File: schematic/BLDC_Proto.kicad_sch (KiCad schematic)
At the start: 50 parts, among them J1 Motor Encoder In, M1 Hobbywing QuicRun 3650, Q1 GSFN0390, Q2 GSFN0390, Q3 GSFN0390, Q4 GSFN0390, Q5 GSFN0390, Q6 GSFN0390, SW1 SW_Push, SW2 Keypad, U1 ESP32-S3-DevKitC, U2 AP62200TWU, U3 DRV8300D, U4 74HC595, U5 74HC595, U6 BA56-12SURKWA, U7 BA56-12SURKWA

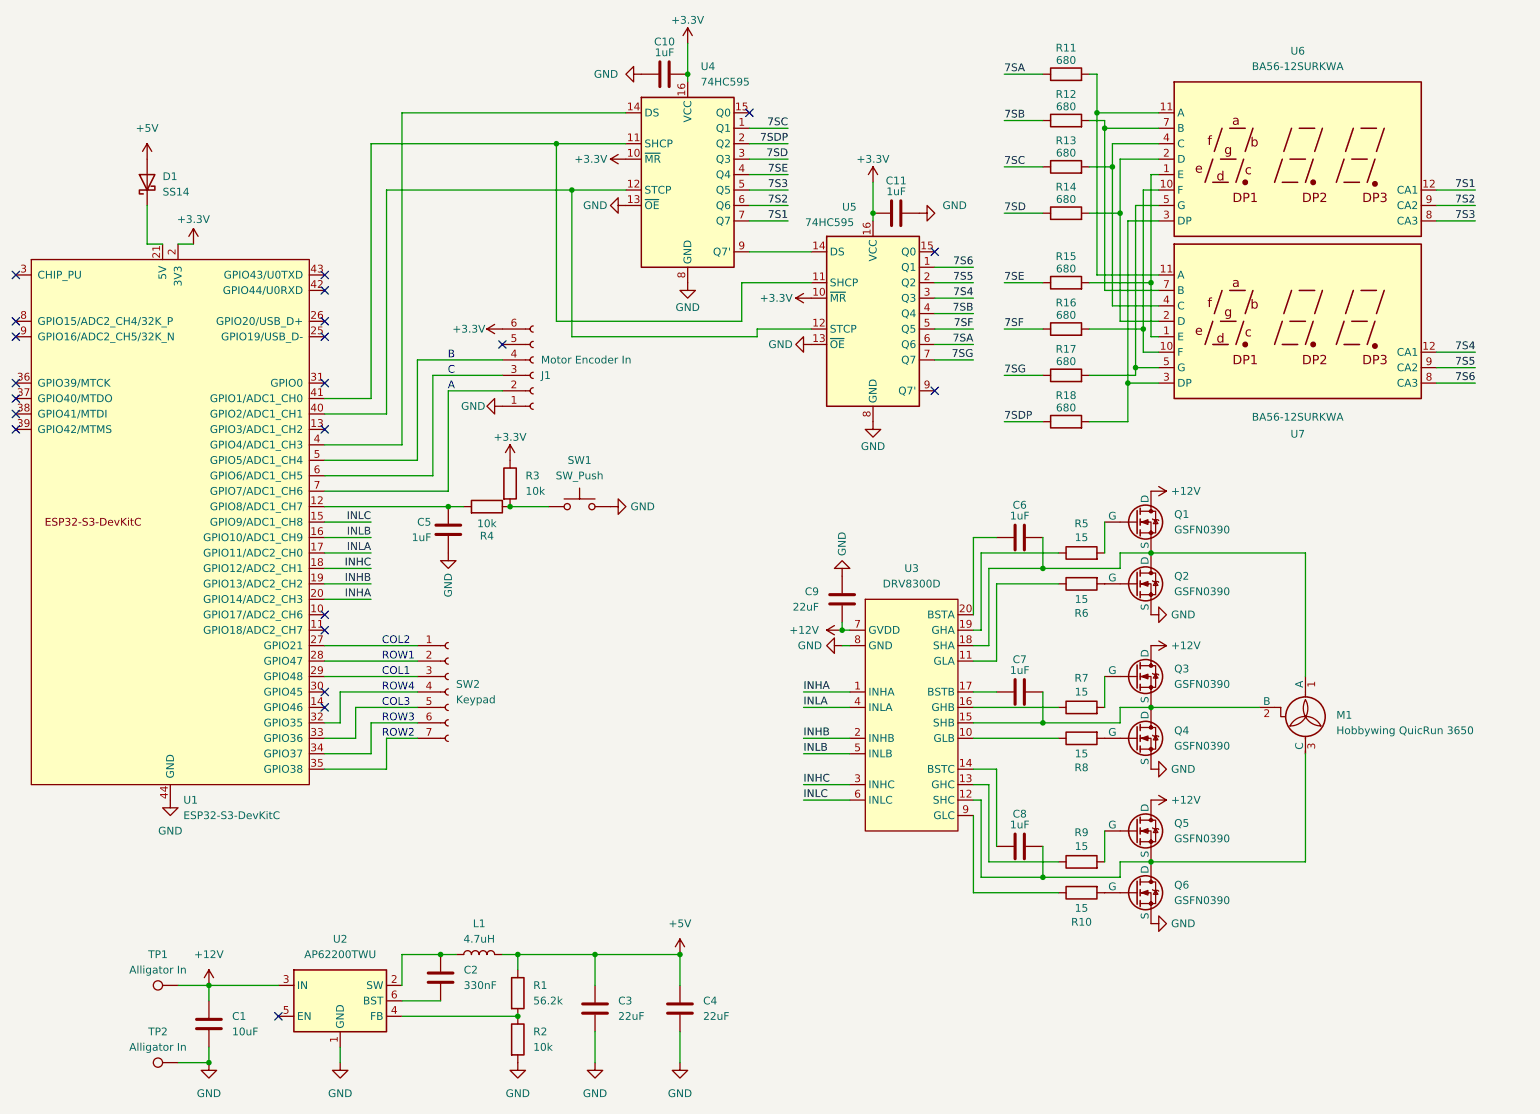
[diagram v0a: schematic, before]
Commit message: 2nd iteration
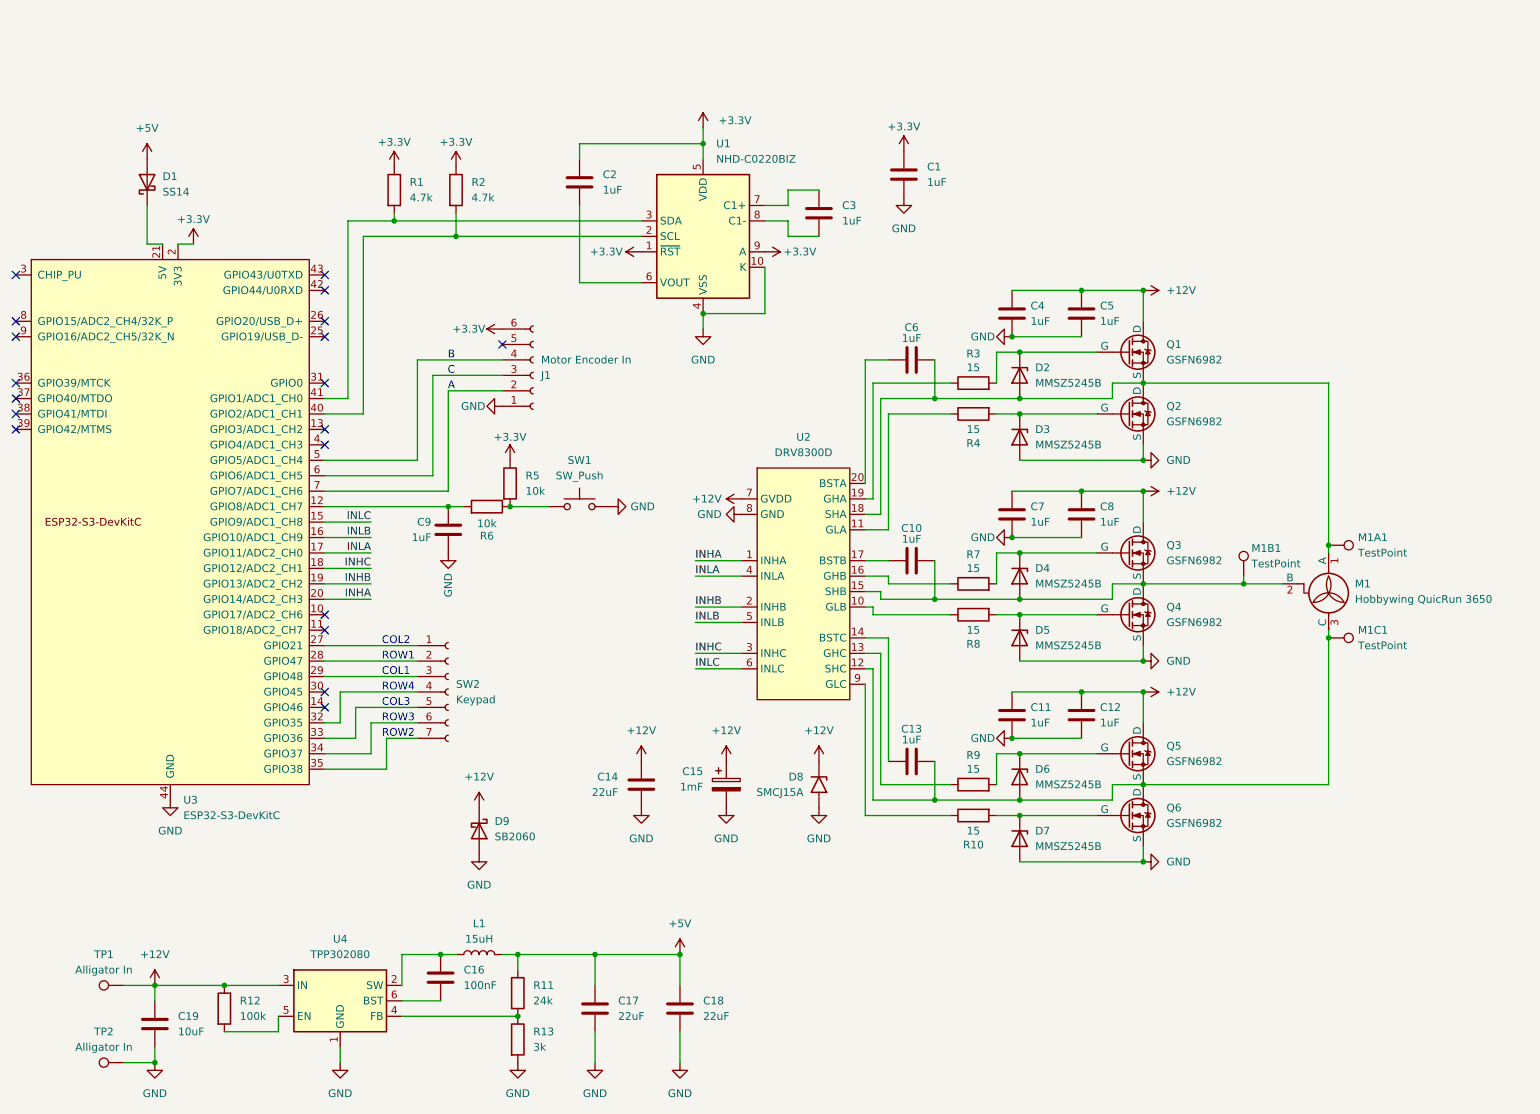
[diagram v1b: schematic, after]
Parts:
- removed C10: 1uF, Capacitor_SMD:C_0805_2012Metric, symbol Device:C
- removed R11, R13, R14, R15, R16, R17, R18: 680, Resistor_SMD:R_0805_2012Metric, symbol Device:R
- removed R5, R6: 15, Resistor_SMD:R_0805_2012Metric, symbol Device:R
- removed U4, U5: 74HC595, Package_SO:TSSOP-16_4.4x5mm_P0.65mm, symbol 74xx:74HC595
- removed U6, U7: BA56-12SURKWA, footprints:BA56-12SURKWA, symbol symbols:LTC-571HR
- added C1, C12, C13, C2, C3, C4, C5, C7: 1uF, Capacitor_SMD:C_0805_2012Metric, symbol Device:C
- added C15: 1mF, Capacitor_THT:CP_Radial_D13.0mm_P5.00mm, symbol Device:C_Polarized
- added D2, D3, D4, D5, D6, D7: MMSZ5245B, Diode_SMD:D_SOD-123, symbol Device:D_Zener
- added D8: SMCJ15A, Diode_SMD:D_SMC, symbol Diode:1.5SMCxxA
- added D9: SB2060, Diode_THT:D_DO-201AD_P15.24mm_Horizontal, symbol Device:D_Schottky
- added M1A1, M1B1, M1C1: TestPoint, footprints:TestPoint_THTPad_D5.0mm_Drill3.0mm, symbol Connector:TestPoint
- added R1, R2: 4.7k, Resistor_SMD:R_0805_2012Metric, symbol Device:R
- added R3, R4: 15, Resistor_SMD:R_0805_2012Metric, symbol Device:R
- added U1: NHD-C0220BIZ, Display:NHD-C0220BiZ, symbol Display_Character:NHD-C0220BIZ
- C16: renamed from C2; value 330nF -> 100nF
- L1: value 4.7uH -> 15uH; footprint footprints:Inductor_2424 -> footprints:HCM1A0805V3-150R
- M1: footprint footprints:BLDC -> (none)
- Q1, Q2, Q3, Q4, Q5, Q6: value GSFN0390 -> GSFN6982
- R11: renamed from R1; value 56.2k -> 24k
- R12: value 680 -> 100k
- R13: renamed from R2; value 10k -> 3k
- U4: renamed from U2; value AP62200TWU -> TPP302080
- renumbered C7 to C10, C9 to C14, C3 to C17, C4 to C18, C1 to C19, C5 to C9, R3 to R5, R4 to R6, U3 to U2, U1 to U3
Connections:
- net 7SB is gone; now on net +12V: R12.1
- net +12V: now also C11.1, C14.1, C8.1, C12.1, C15.1, C4.1, C5.1, C7.1, D8.1 (A1), D9.1 (K); no longer C14.2
- net +3.3V: now also C1.1, C2.1, R1.1, R2.1, U1.1 (~{RST}), U1.5 (VDD), U1.9 (A); no longer C11.2
- net GND: now also C11.2, C14.2, C8.2, C1.2, C12.2, C15.2, C4.2, C5.2, C7.2, D3.2 (A), D5.2 (A), D7.2 (A), D8.2 (A2), D9.2 (A), U1.10 (K), U1.4 (VSS); no longer C11.1, C14.1
- net at C6.2, M1.1 (A), Q1.1 (S)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: now also D2.2 (A), M1A1.1
- net at Q1.4 (G): now also D2.1 (K), R3.2
- net at C10.2, M1.2 (B), Q3.1 (S)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: now also D4.2 (A), M1B1.1
- net at Q3.4 (G), R7.2: now also D4.1 (K)
- net at R12.2: now also U4.5 (EN)
- net at U2.11 (GLA): now also R4.1
- net at M1.3 (C), Q5.1 (S), Q5.2 (S)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: now also C13.2, D6.2 (A), M1C1.1; no longer C8.2
- net at U2.14 (BSTC): now also C13.1; no longer C8.1
- net at U2.19 (GHA): now also R3.1
- net at Q6.4 (G), R10.2: now also D7.1 (K)
- net at Q4.4 (G), R8.2: now also D5.1 (K)
- net at U3.41 (GPIO1/ADC1_CH0): now also R1.2, U1.3 (SDA)
- net at U3.40 (GPIO2/ADC1_CH1): now also R2.2, U1.2 (SCL)
- net at Q2.4 (G): now also D3.1 (K), R4.2
- net at Q5.4 (G), R9.2: now also D6.1 (K)
- new net: C2.2, U1.6 (VOUT)
- new net: C3.1, U1.7 (C1+)
- new net: C3.2, U1.8 (C1-)
- no-connect marks 22 -> 19
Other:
- moved on the sheet: C10, C14, C19, M1, Q3, R7, R8, TP1, TP2, U2
